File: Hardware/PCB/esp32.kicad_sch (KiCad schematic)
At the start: 6 parts, among them U1 ESP32-S3-WROOM-1

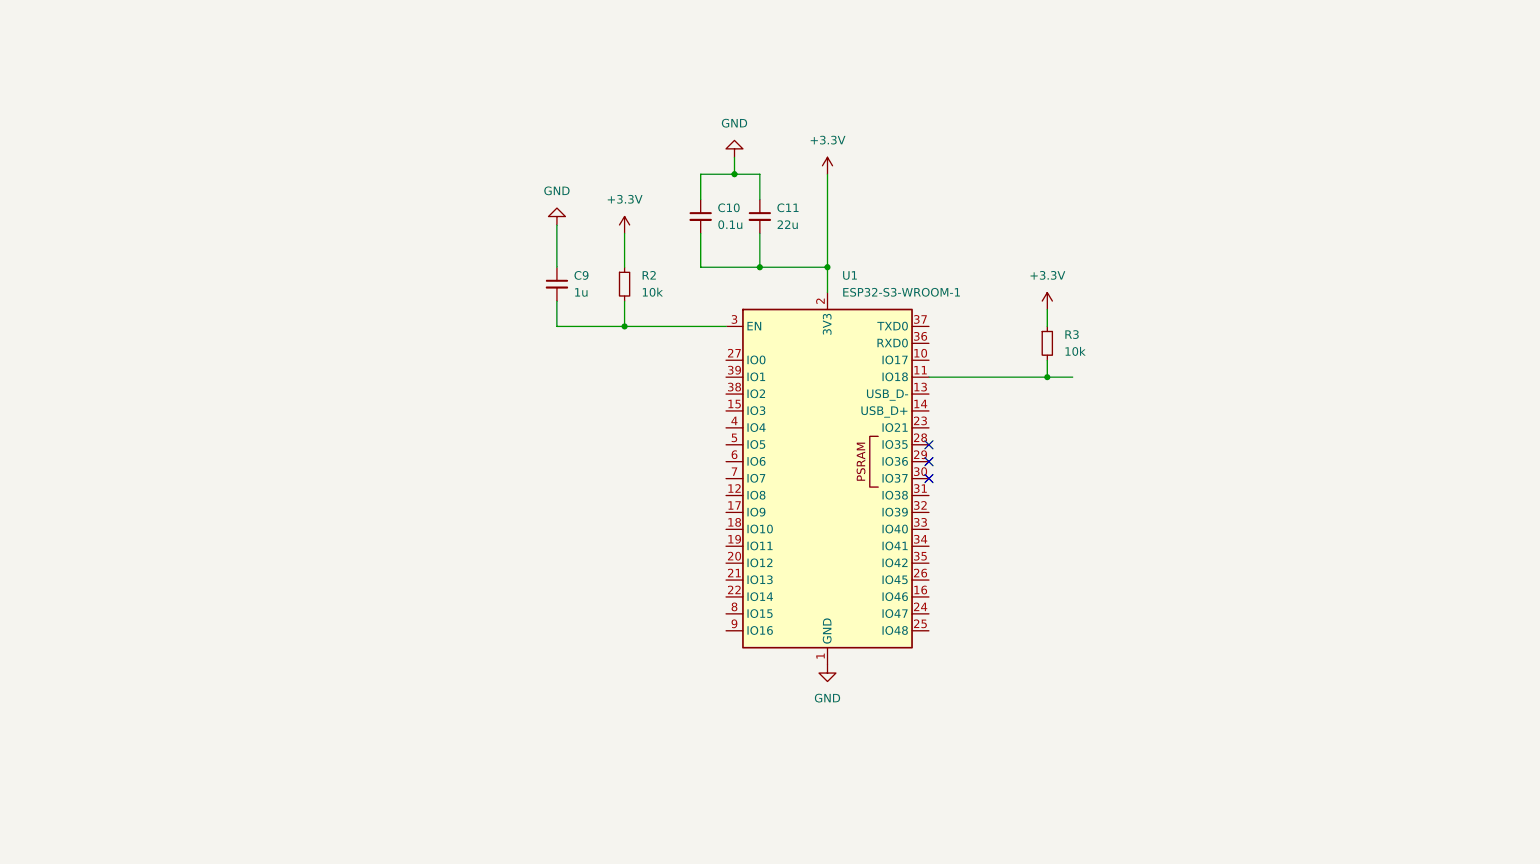
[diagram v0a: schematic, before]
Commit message: added a lot of stuff, going to work on LCD + Touch next
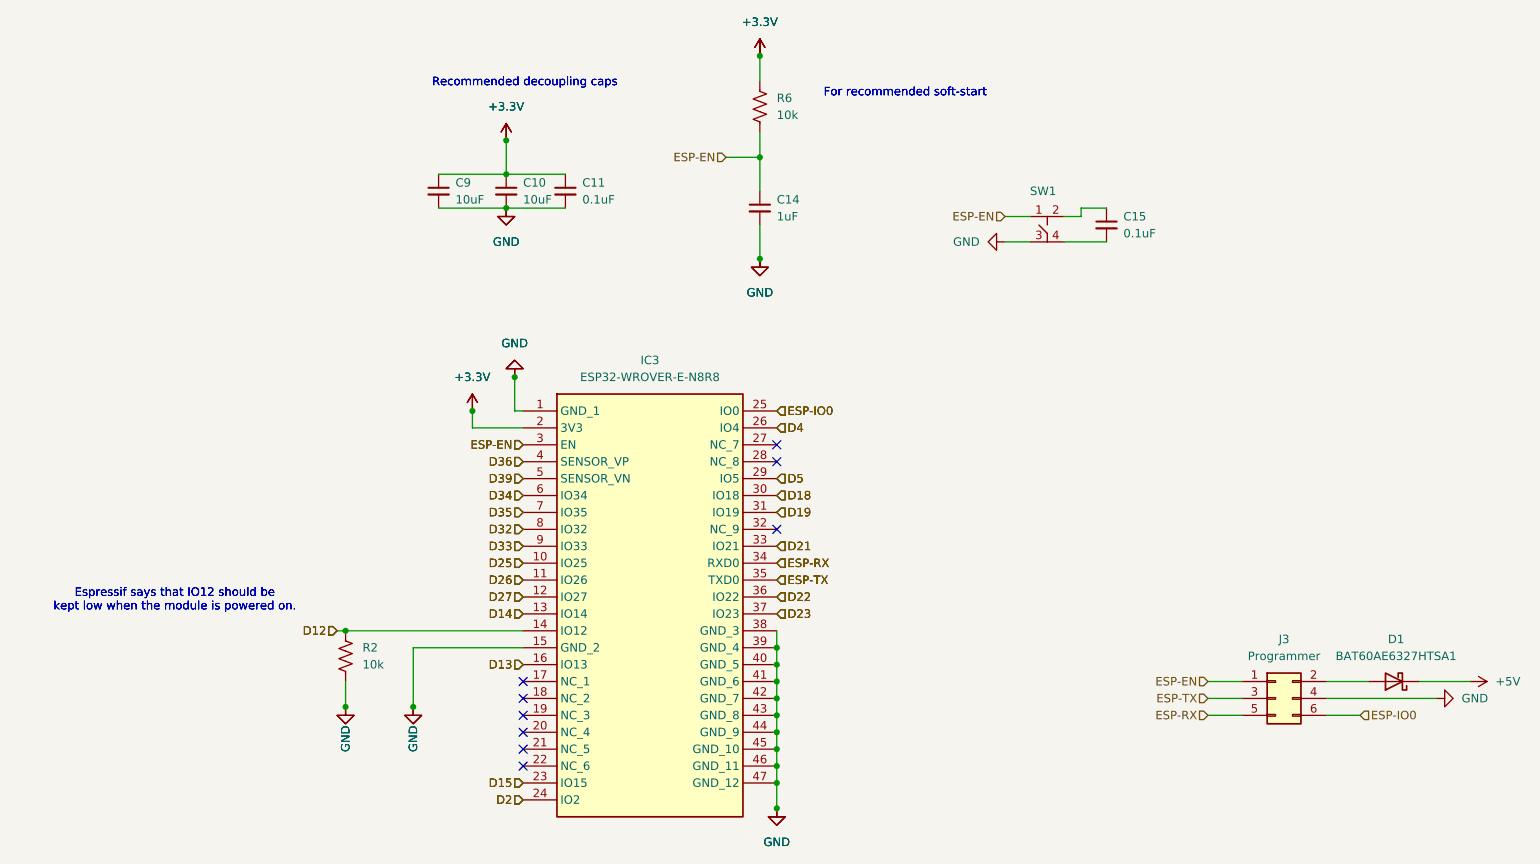
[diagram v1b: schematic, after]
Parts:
- removed R2, R3: 10k, Resistor_SMD:R_0603_1608Metric_Pad0.98x0.95mm_HandSolder, symbol Device:R_Small
- removed U1: ESP32-S3-WROOM-1, RF_Module:ESP32-S3-WROOM-1, symbol RF_Module:ESP32-S3-WROOM-1
- added C14: 1uF, Capacitor_SMD:C_0805_2012Metric_Pad1.18x1.45mm_HandSolder, symbol Device:C_Small
- added C15: 0.1uF, Capacitor_SMD:C_0603_1608Metric_Pad1.08x0.95mm_HandSolder, symbol Device:C_Small
- added D1: BAT60AE6327HTSA1, Diode_SMD:D_SOD-323_HandSoldering, symbol Device:D_Schottky
- added IC3: ESP32-WROVER-E-N8R8, Custom Footprints:ESP32WROVEREN8R8, symbol Custom Symbols:ESP32-WROVER-E-N8R8
- added J3: Programmer, Vendor_Footprints:61200621621, symbol Connector_Generic:Conn_02x03_Odd_Even
- added R2, R6: 10k, Resistor_SMD:R_0603_1608Metric_Pad0.98x0.95mm_HandSolder, symbol Device:R_US
- added SW1: ~, Vendor_Footprints:PTS647SN50SMTR2LFS, symbol Vendor_Symbols:PTS647SN50SMTR2_LFS
- C10: value 0.1u -> 10uF; footprint Capacitor_SMD:C_0603_1608Metric_Pad1.08x0.95mm_HandSolder -> Capacitor_SMD:C_0805_2012Metric; DigiKey Link (none) -> https://www.digikey.com/en/products/detail/samsung-electro-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; MPN (none) -> GRM21BR61H106KE43L; Manufacturer (none) -> Murata Electronics
- C11: value 22u -> 0.1uF; footprint Capacitor_SMD:C_0603_1608Metric_Pad1.08x0.95mm_HandSolder -> Capacitor_SMD:C_0805_2012Metric_Pad1.18x1.45mm_HandSolder; DigiKey Link (none) -> https://www.digikey.com/en/products/detail/samsung-electro-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; MPN (none) -> CL21B104KBCNFNC; Manufacturer (none) -> Samsung Electro-Mechanics
- C9: value 1u -> 10uF; footprint Capacitor_SMD:C_0603_1608Metric_Pad1.08x0.95mm_HandSolder -> Capacitor_SMD:C_0805_2012Metric; DigiKey Link (none) -> https://www.digikey.com/en/products/detail/samsung-electro-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; MPN (none) -> GRM21BR61H106KE43L; Manufacturer (none) -> Murata Electronics
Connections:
- net +3.3V: now also C10.1, C11.1, C9.1, IC3.2 (3V3), R6.1; no longer C10.2, C11.2
- net GND: now also C10.2, C11.2, C9.2, C14.2, IC3.1 (GND_1), IC3.15 (GND_2), IC3.38 (GND_3), IC3.39 (GND_4), IC3.40 (GND_5), IC3.41 (GND_6), IC3.42 (GND_7), IC3.43 (GND_8), IC3.44 (GND_9), IC3.45 (GND_10), IC3.46 (GND_11), IC3.47 (GND_12), J3.4 (Pin_4), R2.2, SW1.3; no longer C10.1, C11.1, C9.1
- new net: D1.2 (A), J3.2 (Pin_2)
- new net: C15.1, SW1.2
- new net: C15.2, SW1.4
- new net +5V: D1.1 (K)
- new net D12: IC3.14 (IO12), R2.1
- new net D13: IC3.16 (IO13)
- new net D14: IC3.13 (IO14)
- new net D15: IC3.23 (IO15)
- new net D18: IC3.30 (IO18)
- new net D19: IC3.31 (IO19)
- new net D2: IC3.24 (IO2)
- new net D21: IC3.33 (IO21)
- new net D22: IC3.36 (IO22)
- new net D23: IC3.37 (IO23)
- new net D25: IC3.10 (IO25)
- new net D26: IC3.11 (IO26)
- new net D27: IC3.12 (IO27)
- new net D32: IC3.8 (IO32)
- new net D33: IC3.9 (IO33)
- new net D34: IC3.6 (IO34)
- new net D35: IC3.7 (IO35)
- new net D36: IC3.4 (SENSOR_VP)
- new net D39: IC3.5 (SENSOR_VN)
- new net D4: IC3.26 (IO4)
- new net D5: IC3.29 (IO5)
- new net ESP-EN: C14.1, IC3.3 (EN), J3.1 (Pin_1), R6.2, SW1.1
- new net ESP-IO0: IC3.25 (IO0), J3.6 (Pin_6)
- new net ESP-RX: IC3.34 (RXD0), J3.5 (Pin_5)
- new net ESP-TX: IC3.35 (TXD0), J3.3 (Pin_3)
- no-connect marks 3 -> 9
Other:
- note added: "Espressif says that IO12 should be kept low when the module is powered on."
- note added: "For recommended soft-start"
- note added: "Recommended decoupling caps"
